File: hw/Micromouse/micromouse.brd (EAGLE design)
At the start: 60 x 97 mm, 54 parts, among them IC1 DSPIC33FJ64MC804-PT, IC2 DRV8833PWR, J1 GP2Y0A51SK0F, J2 GP2Y0A51SK0F, J3 GP2Y0A41SK0F, SW1 B3F-1000

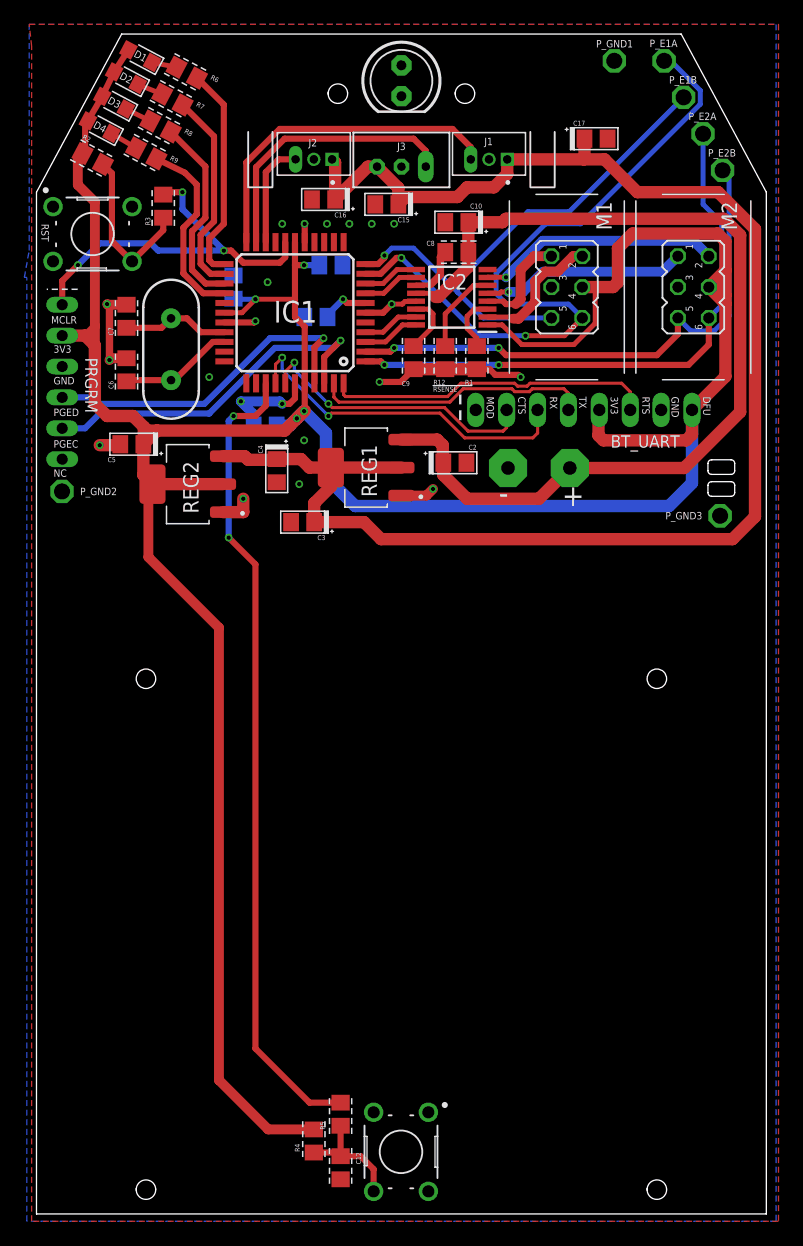
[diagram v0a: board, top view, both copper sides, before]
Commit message: Finalized board; Added speedy gonzales in the process!
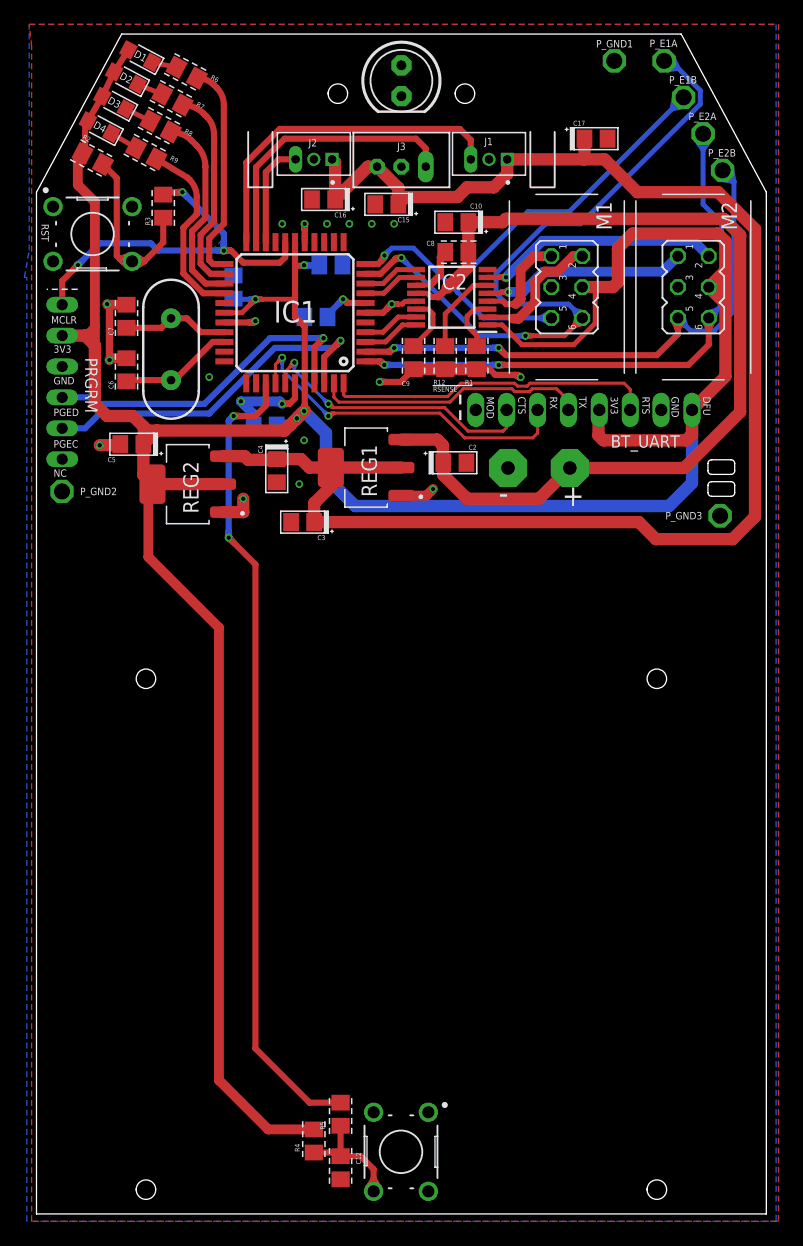
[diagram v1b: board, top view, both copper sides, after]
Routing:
- net M2_CHB: track 45.5 -> 59.1 mm
- net M1_CHA: track 58.8 -> 72.5 mm
- net M2_CHA: track 47.4 -> 60.8 mm
- net M1_CHB: track 45.4 -> 54.0 mm
- net MCLR: track 31.5 -> 39.8 mm
- net GND: track 44.4 -> 52.5 mm, vias 21 -> 20
- net N$7: track 13.6 -> 20.2 mm
- net +3V3: track 260.7 -> 266.8 mm
- net UART_RX: track 28.9 -> 34.4 mm
- net BT_CTS: track 23.7 -> 29.2 mm
- net SW1: track 66.8 -> 71.5 mm
- net OSC2: track 9.39 -> 13.3 mm
- net OSC1: track 8.85 -> 12.7 mm
- net N$6: track 9.81 -> 12.6 mm
- net PGED3: track 28.0 -> 30.3 mm
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- added copper zone on layer 16, net MCLR
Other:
- board text added: "MICROMOUSE WISE20/21"
- board text added: "Philipp Hagenlocher Matteo Nardini Hendrik Möller Congnan Wang"
